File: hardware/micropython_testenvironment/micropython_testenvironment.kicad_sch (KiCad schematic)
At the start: 12 parts, among them J101 Conn_01x16, J102 Conn_01x16, J103 Conn_01x16, J104 Conn_01x16, J105 Conn_01x16, J106 Conn_01x16, J107 Conn_01x16, J108 Conn_01x16, J109 Conn_01x16, SW101 SW_Push, SW102 SW_Push, SW103 SW_Push

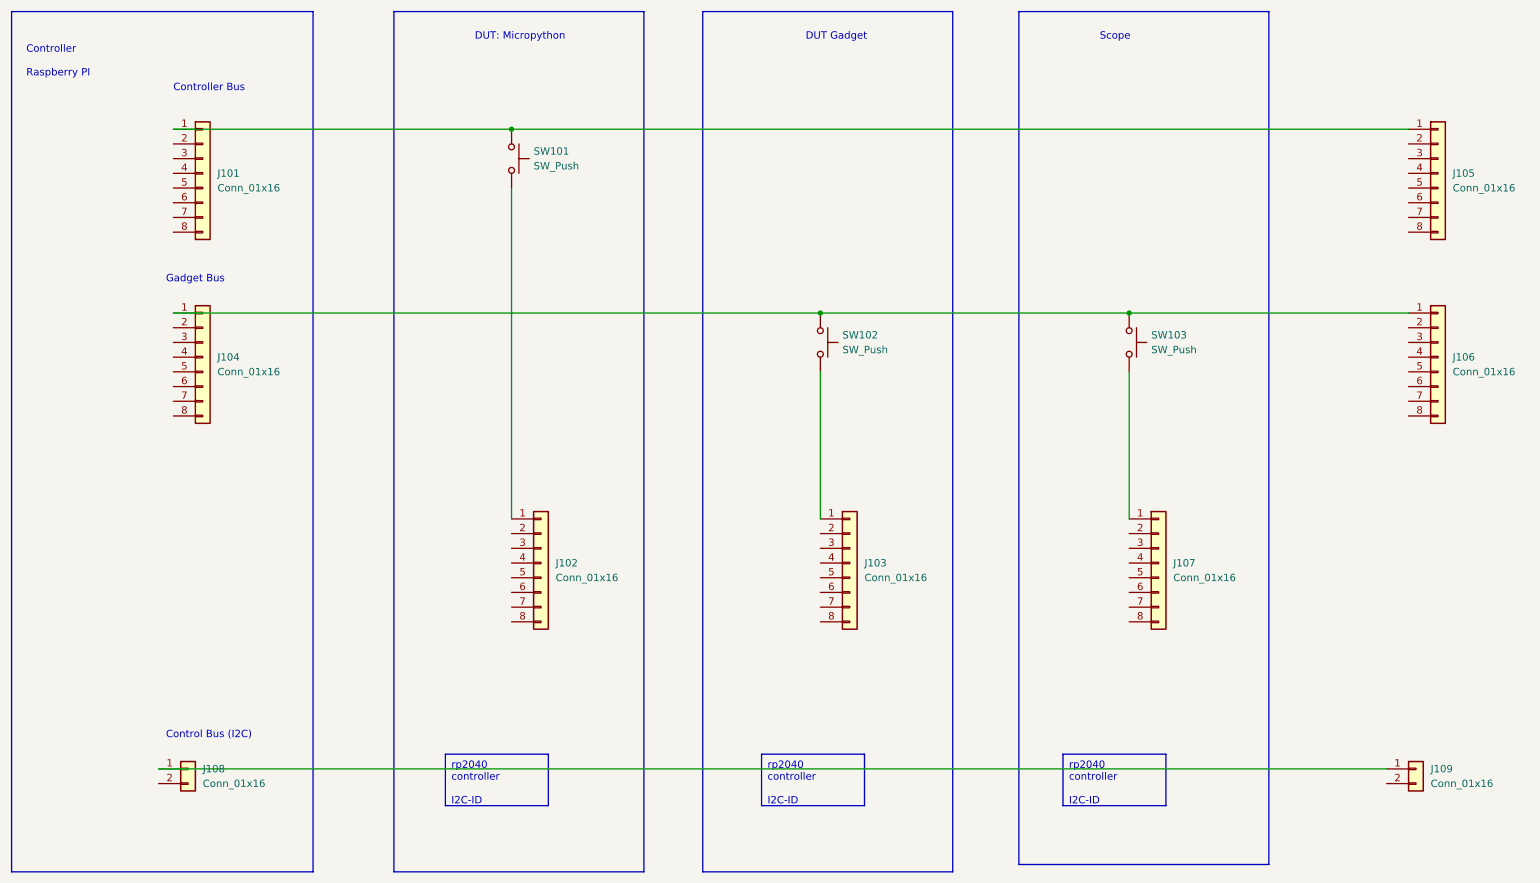
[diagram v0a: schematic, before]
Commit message: Initial ideas 2
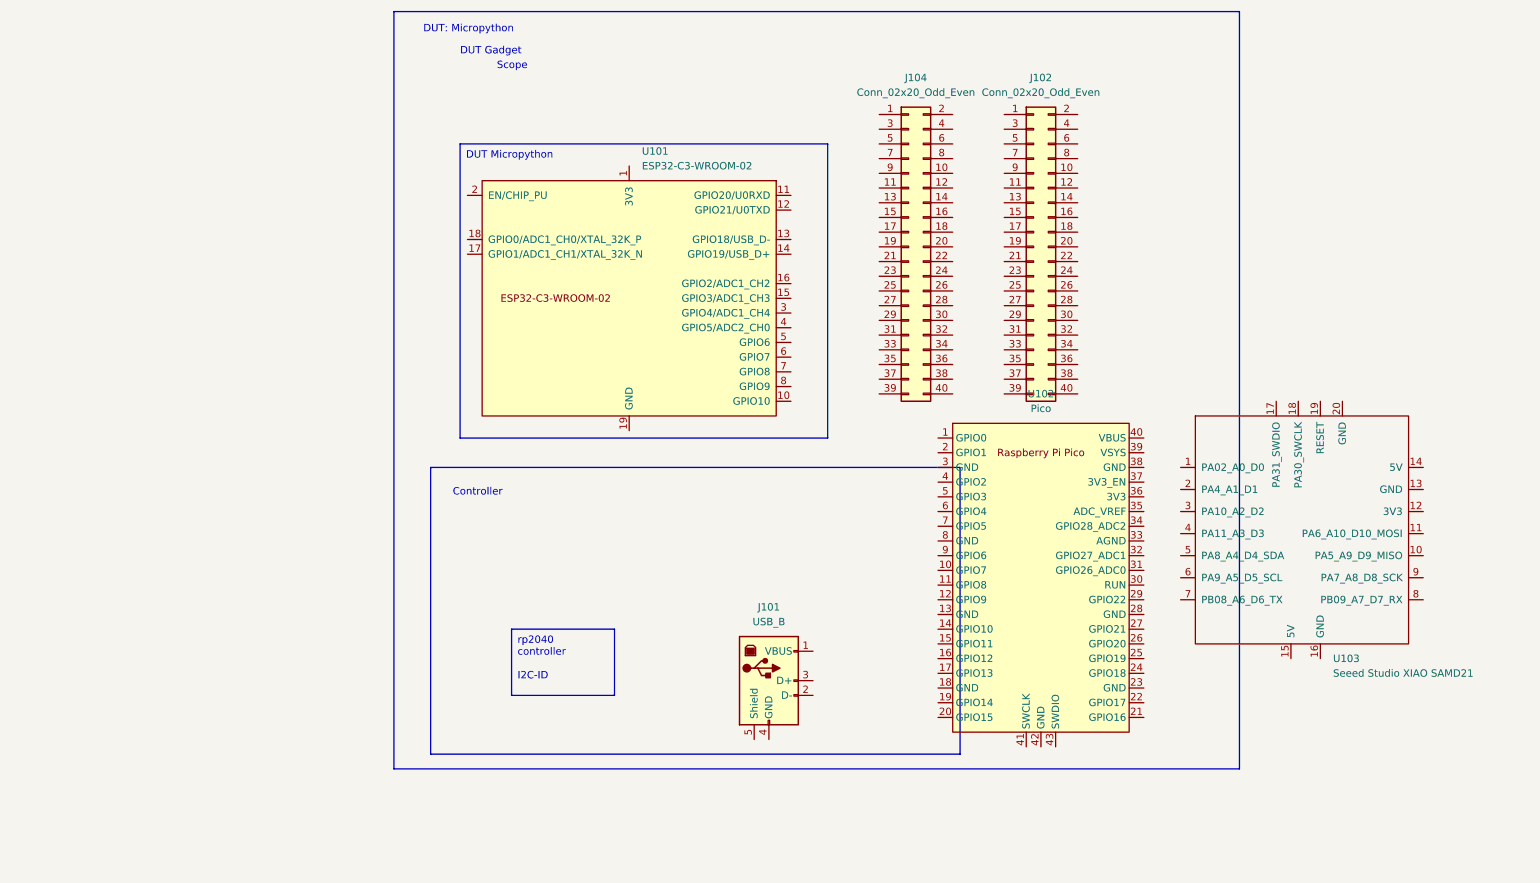
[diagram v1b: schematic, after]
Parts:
- removed J101, J102, J103, J104, J105, J106, J107: Conn_01x16, symbol Connector_Generic:Conn_01x08
- removed J108, J109: Conn_01x16, symbol Connector_Generic:Conn_01x02
- removed SW101, SW102, SW103: SW_Push, symbol Switch:SW_Push
- added J101: USB_B, symbol Connector:USB_B
- added J102: Conn_02x20_Odd_Even, Connector_PinSocket_2.54mm:PinSocket_2x20_P2.54mm_Vertical, symbol Connector_Generic:Conn_02x20_Odd_Even
- added J104: Conn_02x20_Odd_Even, Connector_PinHeader_2.54mm:PinHeader_2x20_P2.54mm_Vertical, symbol Connector_Generic:Conn_02x20_Odd_Even
- added U101: ESP32-C3-WROOM-02, PCM_Espressif:ESP32-C3-WROOM-02, symbol PCM_Espressif:ESP32-C3-WROOM-02
- added U102: Pico, 00_project_library:RPi_Pico_SMD_TH, symbol 00_project_library:Pico
- added U103: Seeed Studio XIAO SAMD21, 00_project_library:XIAO-SAMD21-RP2040-14P-2.54-21X17.8MM (Seeeduino XIAO), symbol 00_project_library:Seeed Studio XIAO SAMD21
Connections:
- new net: U101.19 (GND), U101.9 (GND)
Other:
- note added: "Controller"
- note removed: "Control Bus (I2C)"
- note removed: "Controller Bus"
- note removed: "Controller Raspberry PI"
- note removed: "Gadget Bus"
